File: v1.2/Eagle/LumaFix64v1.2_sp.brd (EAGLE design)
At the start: 25.9 x 50.8 mm, 16 parts, among them IC1 74HCT14D

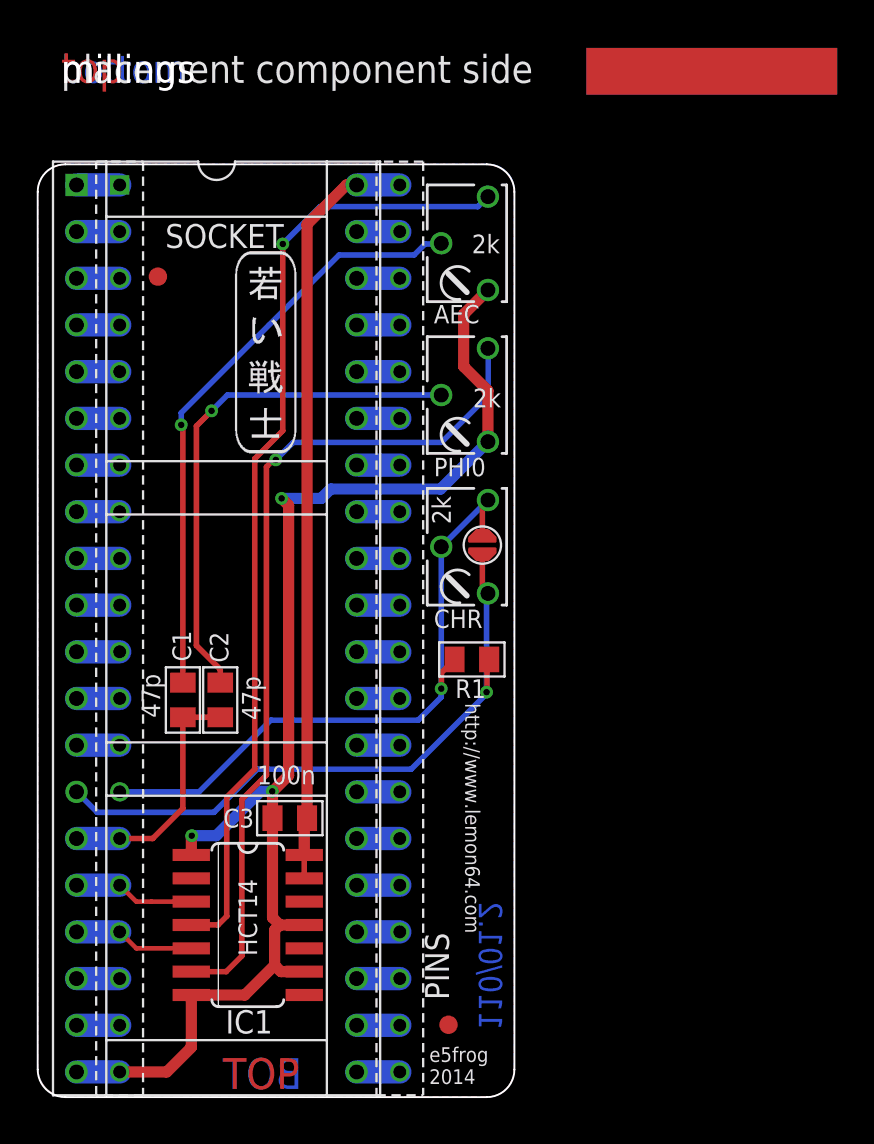
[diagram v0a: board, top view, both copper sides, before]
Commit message: Silk Screen Update
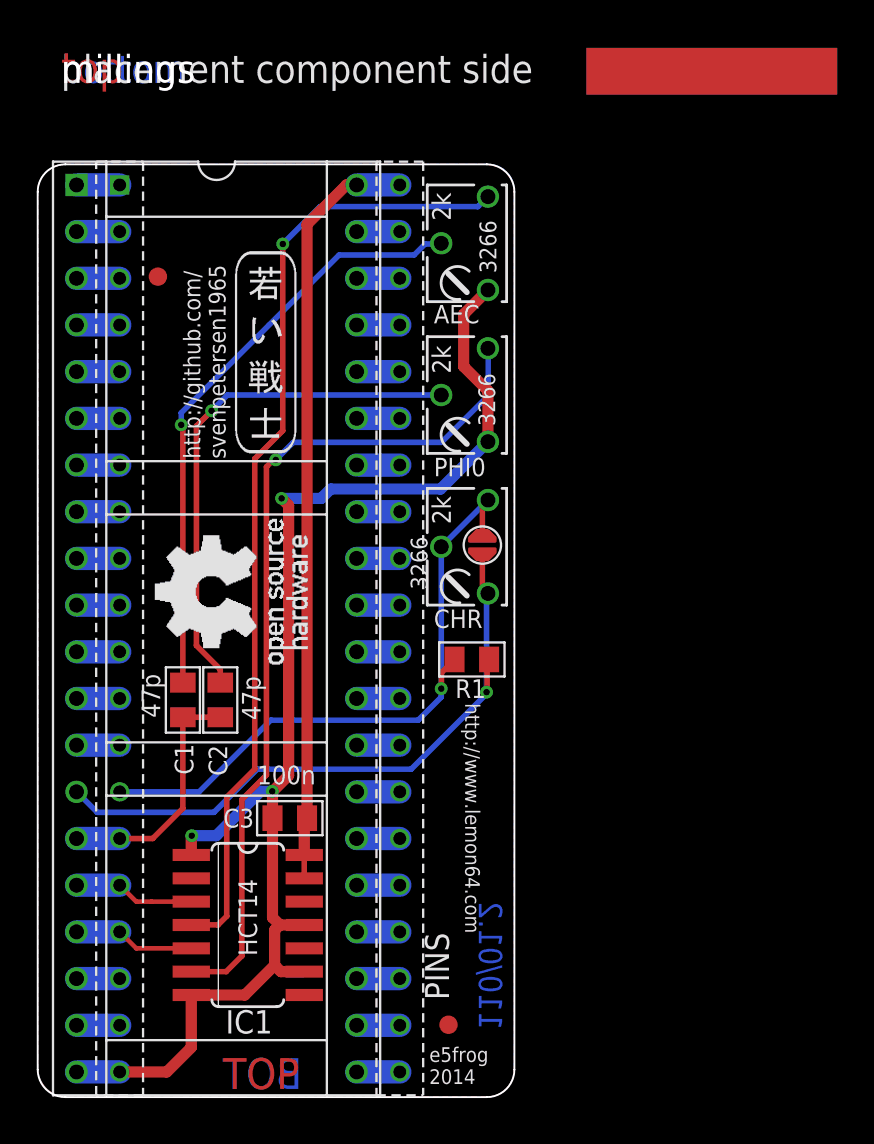
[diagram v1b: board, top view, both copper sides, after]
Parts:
- added U$13: OPEN_SOURCE_HW, Logo:OPENHW
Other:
- board text added: "3266"
- board text added: "http://github.com/ svenpetersen1965"
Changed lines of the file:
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@@
 <grid distance="0.0635" unitdist="mm" unit="mil" style="dots" multiple="1" display="no" altdistance="0.0125" altunitdist="inch" altunit="mil"/>
 <layers>
-<layer number="1" name="Top" color="4" fill="1" visible="yes" active="yes"/>
+<layer number="1" name="Top" color="4" fill="1" visible="no" active="yes"/>
 <layer number="2" name="Route2" color="1" fill="3" visible="no" active="no"/>
 <layer number="3" name="Route3" color="4" fill="3" visible="no" active="no"/>
@@
 <layer number="14" name="Route14" color="1" fill="6" visible="no" active="no"/>
 <layer number="15" name="Route15" color="4" fill="6" visible="no" active="no"/>
-<layer number="16" name="Bottom" color="1" fill="1" visible="yes" active="yes"/>
-<layer number="17" name="Pads" color="2" fill="1" visible="yes" active="yes"/>
-<layer number="18" name="Vias" color="2" fill="1" visible="yes" active="yes"/>
+<layer number="16" name="Bottom" color="1" fill="1" visible="no" active="yes"/>
+<layer number="17" name="Pads" color="2" fill="1" visible="no" active="yes"/>
+<layer number="18" name="Vias" color="2" fill="1" visible="no" active="yes"/>
 <layer number="19" name="Unrouted" color="6" fill="1" visible="yes" active="yes"/>
 <layer number="20" name="Dimension" color="15" fill="1" visible="yes" active="yes"/>
 <layer number="21" name="tPlace" color="7" fill="1" visible="yes" active="yes"/>
 <layer number="22" name="bPlace" color="7" fill="1" visible="no" active="yes"/>
-<layer number="23" name="tOrigins" color="15" fill="1" visible="yes" active="yes"/>
+<layer number="23" name="tOrigins" color="15" fill="1" visible="no" active="yes"/>
 <layer number="24" name="bOrigins" color="15" fill="1" visible="no" active="yes"/>
 <layer number="25" name="tNames" color="7" fill="1" visible="yes" active="yes"/>
@@
 <layer number="27" name="tValues" color="7" fill="1" visible="no" active="yes"/>
 <layer number="28" name="bValues" color="7" fill="1" visible="no" active="yes"/>
-<layer number="29" name="tStop" color="7" fill="3" visible="yes" active="yes"/>
+<layer number="29" name="tStop" color="7" fill="3" visible="no" active="yes"/>
 <layer number="30" name="bStop" color="7" fill="6" visible="no" active="yes"/>
 <layer number="31" name="tCream" color="7" fill="4" visible="no" active="yes"/>
@@
 <layer number="45" name="Holes" color="7" fill="1" visible="no" active="yes"/>
 <layer number="46" name="Milling" color="3" fill="1" visible="no" active="yes"/>
-<layer number="47" name="Measures" color="7" fill="1" visible="yes" active="yes"/>
+<layer number="47" name="Measures" color="7" fill="1" visible="no" active="yes"/>
 <layer number="48" name="Document" color="5" fill="1" visible="yes" active="yes"/>
 <layer number="49" name="Reference" color="7" fill="1" visible="no" active="yes"/>
@@
 <layer number="250" name="Descript" color="7" fill="1" visible="no" active="no"/>
 <layer number="251" name="SMDround" color="7" fill="1" visible="no" active="no"/>
+<layer number="252" name="BR-BS" color="7" fill="1" visible="no" active="yes"/>
+<layer number="253" name="BR-LS" color="7" fill="1" visible="no" active="yes"/>
 <layer number="254" name="OrgLBR" color="7" fill="1" visible="no" active="no"/>
 <layer number="255" name="Accent" color="7" fill="1" visible="yes" active="yes"/>
@@
 <text x="11.938" y="7.6835" size="1.016" layer="21" font="vector" ratio="12" rot="R90">HCT14</text>
 <text x="11.938" y="17.018" size="1.016" layer="21" font="vector" ratio="12">100n</text>
-<text x="23.622" y="45.9105" size="1.016" layer="21" font="vector" ratio="12">2k</text>
-<text x="23.6855" y="37.5285" size="1.016" layer="21" font="vector" ratio="12">2k</text>
+<text x="22.479" y="47.6885" size="1.016" layer="21" font="vector" ratio="12" rot="R90">2k</text>
+<text x="22.479" y="39.37" size="1.016" layer="21" font="vector" ratio="12" rot="R90">2k</text>
 <text x="22.479" y="31.1785" size="1.016" layer="21" font="vector" ratio="12" rot="R90">2k</text>
+<text x="10.2235" y="34.7345" size="0.9144" layer="21" ratio="12" rot="R90">http://github.com/
+svenpetersen1965</text>
+<text x="24.9555" y="44.831" size="0.9144" layer="21" ratio="12" rot="R90">3266</text>
+<text x="24.892" y="36.5125" size="0.9144" layer="21" ratio="12" rot="R90">3266</text>
+<text x="21.209" y="27.6225" size="0.9144" layer="21" ratio="12" rot="R90">3266</text>
 </plain>
 <attributes>
@@
 <elements>
 <element name="SOCKET" library="LumaFix64v1.0_B64W" package="GS40P" value="" x="9.73375" y="25.5" smashed="yes" rot="R270">
-<attribute name="NAME" x="6.93975" y="46.201" size="1.3" layer="25" font="vector" ratio="13"/>
 <attribute name="VALUE" x="8.71775" y="42.645" size="1.778" layer="27" rot="R270"/>
 </element>
@@
 </element>
 <element name="C1" library="SMD" package="0805" value="47p" x="7.901" y="21.60825" smashed="yes" rot="R90">
-<attribute name="NAME" x="8.3455" y="23.70375" size="1.016" layer="25" ratio="10" rot="R90"/>
+<attribute name="NAME" x="8.4725" y="17.54425" size="1.016" layer="25" ratio="10" rot="R90"/>
 <attribute name="VALUE" x="8.3455" y="20.02075" size="1.016" layer="27" ratio="10" rot="R90"/>
 </element>
 <element name="C2" library="SMD" package="0805" value="47p" x="9.933" y="21.60825" smashed="yes" rot="R90">
-<attribute name="NAME" x="10.3775" y="23.64025" size="1.016" layer="25" ratio="10" rot="R90"/>
+<attribute name="NAME" x="10.314" y="17.48075" size="1.016" layer="25" ratio="10" rot="R90"/>
 <attribute name="VALUE" x="10.3775" y="20.02075" size="1.016" layer="27" ratio="10" rot="R90"/>
 </element>
@@
 <attribute name="VALUE" x="25.2095" y="24.257" size="1.016" layer="27" ratio="10" rot="R180"/>
 </element>
+<element name="U$13" library="Logo" package="OPENHW" value="OPEN_SOURCE_HW" x="14.6685" y="23.5585" smashed="yes" rot="R90"/>
 </elements>
 <signals>
